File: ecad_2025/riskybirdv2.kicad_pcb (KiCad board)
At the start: 2 copper layers, 58.3 x 58.3 mm, 1 part

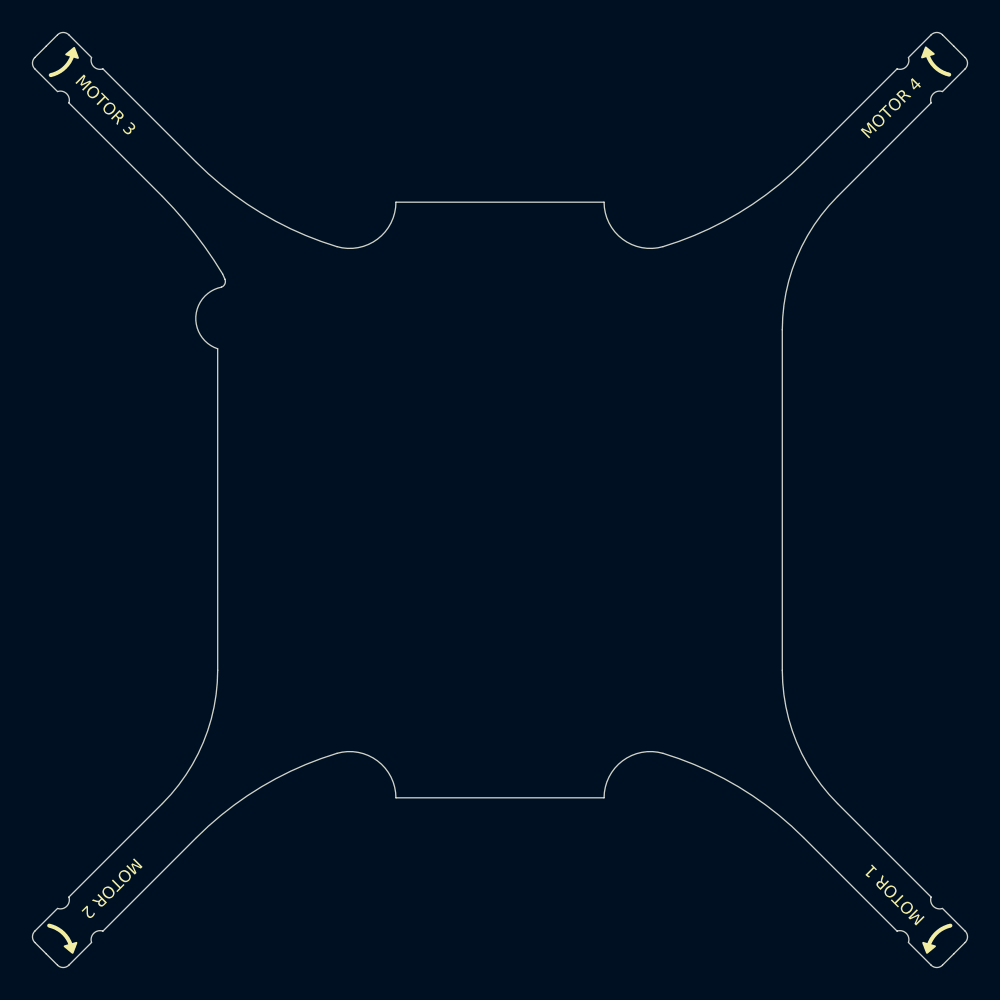
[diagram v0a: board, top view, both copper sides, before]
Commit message: first revision of riskybirdv2 sensor board
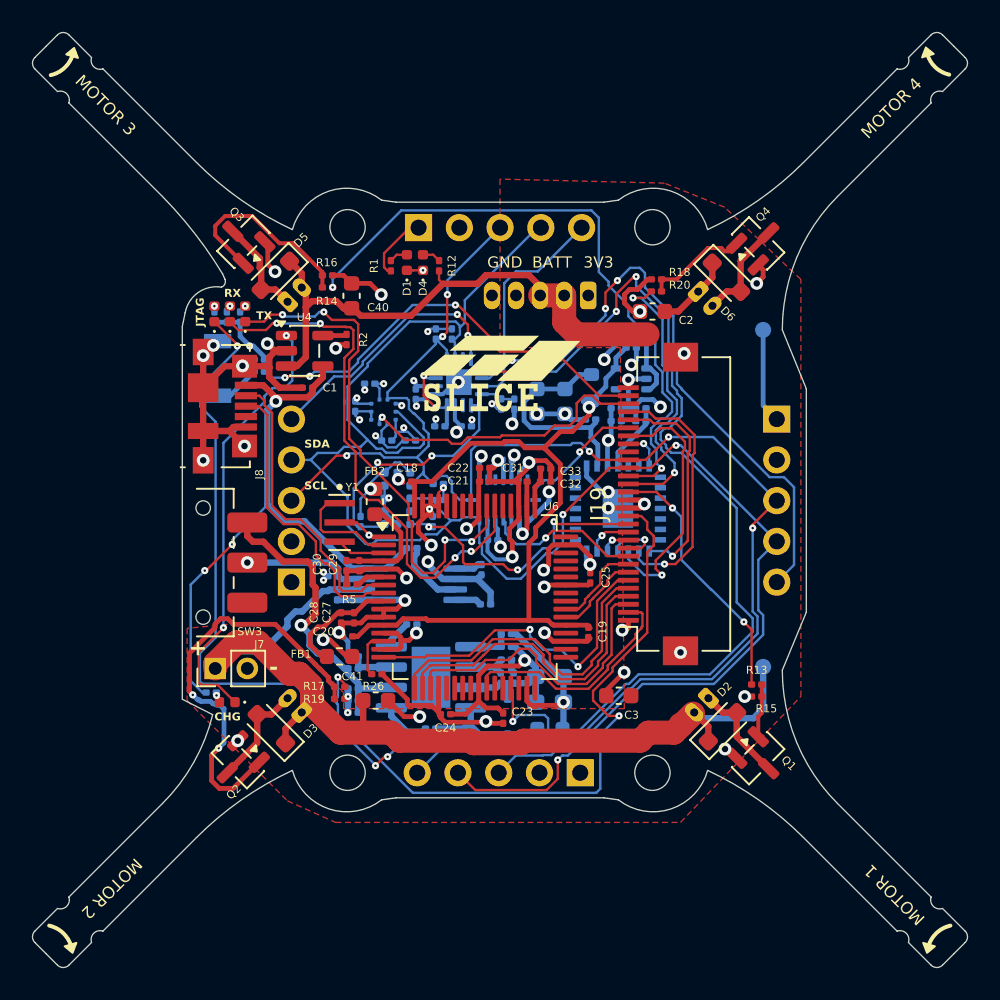
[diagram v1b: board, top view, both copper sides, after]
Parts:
- added C1: 4.7u, Capacitor_SMD:C_0201_0603Metric, F.Cu at (88.0, 93.0)
- added C10: 100nF, Capacitor_SMD:C_0201_0603Metric, B.Cu at (108.8, 95.1)
- added C11: 22uF, Capacitor_SMD:C_0603_1608Metric, B.Cu at (102.3, 93.9)
- added C12: 22uF, Capacitor_SMD:C_0603_1608Metric, B.Cu at (104.0, 93.9)
- added C13: 100nF, Capacitor_SMD:C_0201_0603Metric, B.Cu at (105.6, 95.0)
- added C14: 10uF, Capacitor_SMD:C_0201_0603Metric, B.Cu at (107.2, 95.1)
- added C15: 100nF, Capacitor_SMD:C_0201_0603Metric, B.Cu at (107.2, 94.3)
- added C16: 100n, Capacitor_SMD:C_0201_0603Metric, B.Cu at (91.0, 94.2)
- added C17: 100n, Capacitor_SMD:C_0201_0603Metric, B.Cu at (91.9, 92.8)
- added C18: 100nF, Capacitor_SMD:C_0201_0603Metric, F.Cu at (94.2, 98.8)
- added C19: 100nF, Capacitor_SMD:C_0201_0603Metric, F.Cu at (105.5, 108.2)
- added C2: 47uF, Capacitor_SMD:C_0603_1608Metric, F.Cu at (109.5, 88.2)
- added C20: 100nF, Capacitor_SMD:C_0201_0603Metric, F.Cu at (90.5, 108.5)
- added C21: 100nF, Capacitor_SMD:C_0201_0603Metric, F.Cu at (99.0, 98.8)
- added C22: 100nF, Capacitor_SMD:C_0201_0603Metric, F.Cu at (99.0, 98.0)
- added C23: 10uF, Capacitor_SMD:C_0201_0603Metric, F.Cu at (100.2, 113.6)
- added C24: 100nF, Capacitor_SMD:C_0201_0603Metric, F.Cu at (96.6, 113.3)
- added C25: 100nF, Capacitor_SMD:C_0201_0603Metric, F.Cu at (105.6, 104.8)
- added C26: 4.7u, Capacitor_SMD:C_0201_0603Metric, B.Cu at (89.8, 105.9)
- added C27: 100nF, Capacitor_SMD:C_0201_0603Metric, F.Cu at (90.9, 107.3)
- added C28: 4.7uF, Capacitor_SMD:C_0201_0603Metric, F.Cu at (90.1, 107.3)
- added C29: 100nF, Capacitor_SMD:C_0201_0603Metric, F.Cu at (91.2, 104.1)
- added C3: 47uF, Capacitor_SMD:C_0603_1608Metric, F.Cu at (107.4, 112.2)
- added C30: 4.7uF, Capacitor_SMD:C_0201_0603Metric, F.Cu at (90.4, 104.1)
- added C31: 100nF, Capacitor_SMD:C_0201_0603Metric, F.Cu at (101.4, 98.8)
- added C32: 3.3uF, Capacitor_SMD:C_0201_0603Metric, F.Cu at (102.8, 98.8)
- added C33: 100nF, Capacitor_SMD:C_0201_0603Metric, F.Cu at (102.8, 98.0)
- added C34: 1u, Capacitor_SMD:C_0201_0603Metric, B.Cu at (89.6, 104.8)
- added C38: 100nF, Capacitor_SMD:C_0201_0603Metric, B.Cu at (94.4, 96.3)
- added C39: 4.7uF, Capacitor_SMD:C_0201_0603Metric, B.Cu at (92.9, 96.3)
- added C4: 100nF, Capacitor_SMD:C_0201_0603Metric, B.Cu at (100.4, 97.5)
- added C40: 47uF, Capacitor_SMD:C_0603_1608Metric, F.Cu at (90.8, 87.3)
- added C41: 47uF, Capacitor_SMD:C_0603_1608Metric, F.Cu at (92.2, 112.5)
- added C42: 1uF, Capacitor_SMD:C_0201_0603Metric, B.Cu at (108.2, 90.5)
- added C47: 0.1uF, Capacitor_SMD:C_0201_0603Metric, B.Cu at (95.7, 114.2)
- added C48: 0.01uF, Capacitor_SMD:C_0201_0603Metric, B.Cu at (94.5, 107.8)
- added C49: 1000pF, Capacitor_SMD:C_0201_0603Metric, B.Cu at (100.0, 111.1)
- added C5: 100nF, Capacitor_SMD:C_0201_0603Metric, B.Cu at (99.5, 102.5)
- added C50: 47pF, Capacitor_SMD:C_0201_0603Metric, B.Cu at (100.4, 110.0)
- added C51: 4.7uF, Capacitor_SMD:C_0201_0603Metric, B.Cu at (90.8, 112.5)
- added C52: 47uF, Capacitor_SMD:C_0603_1608Metric_Pad1.08x0.95mm_HandSolder, B.Cu at (103.1, 112.6)
- added C53: 47uF, Capacitor_SMD:C_0603_1608Metric_Pad1.08x0.95mm_HandSolder, B.Cu at (103.1, 111.0)
- added C54: 0.01uF, Capacitor_SMD:C_0201_0603Metric, B.Cu at (90.8, 113.2)
- added C55: 4.7uF, Capacitor_SMD:C_0201_0603Metric, B.Cu at (90.8, 111.8)
- added C6: 100nF, Capacitor_SMD:C_0201_0603Metric, B.Cu at (97.9, 95.4)
- added C7: 100nF, Capacitor_SMD:C_0201_0603Metric, B.Cu at (94.8, 93.4)
- added C8: 1uF, Capacitor_SMD:C_0201_0603Metric, B.Cu at (96.2, 95.4)
- added C9: 4.7uF, Capacitor_SMD:C_0201_0603Metric, B.Cu at (108.8, 94.3)
- added D1: LED, LED_SMD:LED_0402_1005Metric, F.Cu at (94.2, 85.2)
- added D10: LED, LED_SMD:LED_0402_1005Metric, F.Cu at (83.2, 88.4)
- added D11: LED, LED_SMD:LED_0402_1005Metric, F.Cu at (84.1, 88.4)
- added D12: LED, LED_SMD:LED_0402_1005Metric, F.Cu at (82.2, 88.4)
- added D14: BAT54J, Diode_SMD:D_SOD-323F, B.Cu at (100.5, 113.5)
- added D2: BAT54JFILM, Diode_SMD:D_SOD-323_HandSoldering, F.Cu at (113.9, 114.1)
- added D3: BAT54JFILM, Diode_SMD:D_SOD-323_HandSoldering, F.Cu at (85.8, 114.2)
- added D4: LED, LED_SMD:LED_0402_1005Metric, F.Cu at (95.2, 85.2)
- added D5: BAT54JFILM, Diode_SMD:D_SOD-323_HandSoldering, F.Cu at (86.0, 86.0)
- added D6: BAT54JFILM, Diode_SMD:D_SOD-323_HandSoldering, F.Cu at (114.1, 86.1)
- added D7: LED_RED, LED_SMD:LED_0402_1005Metric, F.Cu at (83.0, 112.6)
- added FB1: 600R@100MHz/0.5A, Inductor_SMD:L_0603_1608Metric, F.Cu at (90.0, 109.8)
- added FB2: 600R@100MHz/0.5A, Inductor_SMD:L_0603_1608Metric, F.Cu at (92.2, 100.1)
- added G***: LOGO, LOGO, F.Cu at (100.0, 92.2)
- added G***: LOGO, LOGO, B.Cu at (108.2, 108.8)
- added G***: LOGO, LOGO, B.Cu at (113.8, 99.0)
- added G***: LOGO, LOGO, B.Cu at (92.2, 88.8)
- added H1: MountingHole, MountingHole:MountingHole_2.2mm_M2, F.Cu at (90.5, 83.0)
- added H2: MountingHole, MountingHole:MountingHole_2.2mm_M2, F.Cu at (109.5, 83.0)
- added H3: MountingHole, MountingHole:MountingHole_2.2mm_M2, F.Cu at (90.5, 117.0)
- added H4: MountingHole, MountingHole:MountingHole_2.2mm_M2, F.Cu at (109.5, 117.0)
- added IC1: PMW3901MB-TXQT, riskybird:PMW3901MBTXQT, B.Cu at (107.3, 100.5)
- added J10: Conn_01x05, Connector_PinHeader_2.54mm:PinHeader_1x05_P2.54mm_Vertical, B.Cu at (94.9, 83.0)
- added J11: Conn_01x05, Connector_PinHeader_2.54mm:PinHeader_1x05_P2.54mm_Vertical, B.Cu at (105.0, 117.0)
- added J18: Conn_01x05_MountingPin, Connector_JST:JST_ZH_B5B-ZR_1x05_P1.50mm_Vertical, B.Cu at (105.5, 87.2)
- added J19: Conn_01x30_MountingPin, Connector_FFC-FPC:Hirose_FH12-30S-0.5SH_1x30-1MP_P0.50mm_Horizontal, F.Cu at (109.8, 100.2)
- added J2: Conn_01x05, Connector_PinHeader_2.54mm:PinHeader_1x05_P2.54mm_Vertical, B.Cu at (117.2, 95.0)
- added J3: Conn_01x02, Connector_Molex:Molex_PicoBlade_53048-0210_1x02_P1.25mm_Horizontal, B.Cu at (113.0, 112.4)
- added J4: Conn_01x02, Connector_Molex:Molex_PicoBlade_53048-0210_1x02_P1.25mm_Horizontal, B.Cu at (86.8, 87.6)
- added J5: Conn_01x02, Connector_Molex:Molex_PicoBlade_53048-0210_1x02_P1.25mm_Horizontal, B.Cu at (87.6, 113.2)
- added J6: Conn_01x02, Connector_Molex:Molex_PicoBlade_53048-0210_1x02_P1.25mm_Horizontal, B.Cu at (112.4, 87.0)
- added J7: Conn_01x02, Connector_PinHeader_2.00mm:PinHeader_1x02_P2.00mm_Vertical, F.Cu at (82.2, 110.5)
- added J8: USB_B_Micro, Connector_USB:USB_Micro-B_Molex_47346-0001, F.Cu at (82.7, 94.2)
- added J9: Conn_01x05, Connector_PinHeader_2.54mm:PinHeader_1x05_P2.54mm_Vertical, B.Cu at (87.0, 105.1)
- added L3: 6.8uH, Inductor_SMD:L_0603_1608Metric, B.Cu at (103.1, 114.3)
- added Q1: SI2302, Package_TO_SOT_SMD:SOT-23, F.Cu at (116.1, 116.1)
- added Q2: SI2302, Package_TO_SOT_SMD:SOT-23, F.Cu at (83.7, 116.3)
- added Q3: SI2302, Package_TO_SOT_SMD:SOT-23, F.Cu at (84.0, 83.9)
- added Q4: SI2302, Package_TO_SOT_SMD:SOT-23, F.Cu at (116.1, 84.0)
- added R1: 150, Resistor_SMD:R_0201_0603Metric, F.Cu at (93.2, 85.4)
- added R12: 150, Resistor_SMD:R_0201_0603Metric, F.Cu at (96.2, 85.4)
- added R13: 47R, Resistor_SMD:R_0201_0603Metric, F.Cu at (116.0, 111.5)
- added R14: 47R, Resistor_SMD:R_0201_0603Metric, F.Cu at (89.2, 86.8)
- added R15: 10k, Resistor_SMD:R_0201_0603Metric, F.Cu at (116.0, 112.2)
- added R16: 10k, Resistor_SMD:R_0201_0603Metric, F.Cu at (89.2, 86.0)
- added R17: 47R, Resistor_SMD:R_0201_0603Metric, F.Cu at (90.0, 111.6)
- added R18: 47R, Resistor_SMD:R_0201_0603Metric, F.Cu at (109.8, 87.0)
- added R19: 10k, Resistor_SMD:R_0201_0603Metric, F.Cu at (90.0, 112.4)
- added R2: 2k, Resistor_SMD:R_0201_0603Metric, F.Cu at (90.4, 90.0)
- added R20: 10k, Resistor_SMD:R_0201_0603Metric, F.Cu at (109.8, 86.2)
- added R22: 4.7K, Resistor_SMD:R_0201_0603Metric, B.Cu at (97.0, 89.7)
- added R23: 4.7K, Resistor_SMD:R_0201_0603Metric, B.Cu at (96.0, 89.7)
- added R25: 3, Resistor_SMD:R_0603_1608Metric, B.Cu at (105.7, 93.0)
- added R26: 1k, Resistor_SMD:R_0201_0603Metric, F.Cu at (92.3, 110.8)
- added R27: 150, Resistor_SMD:R_0201_0603Metric, B.Cu at (83.0, 88.6)
- added R28: 150, Resistor_SMD:R_0201_0603Metric, B.Cu at (83.8, 88.6)
- added R29: 150, Resistor_SMD:R_0201_0603Metric, B.Cu at (82.2, 88.6)
- added R3: 150, Resistor_SMD:R_0201_0603Metric, B.Cu at (82.0, 112.0)
- added R30: 200K, Resistor_SMD:R_0201_0603Metric, B.Cu at (100.9, 94.0)
- added R31: 100K, Resistor_SMD:R_0201_0603Metric, B.Cu at (100.1, 94.0)
- added R32: 10K, Resistor_SMD:R_0201_0603Metric, B.Cu at (85.0, 91.2)
- added R33: 100, Resistor_SMD:R_0201_0603Metric, B.Cu at (85.0, 92.0)
- added R34: 10k, Resistor_SMD:R_0201_0603Metric, B.Cu at (94.5, 103.0)
- added R37: 150, Resistor_SMD:R_0201_0603Metric, B.Cu at (99.1, 106.5)
- added R38: 10k, Resistor_SMD:R_0201_0603Metric, B.Cu at (98.8, 104.3)
- added R41: 10k, Resistor_SMD:R_0201_0603Metric, B.Cu at (95.8, 101.3)
- added R42: 10k, Resistor_SMD:R_0201_0603Metric, B.Cu at (91.3, 101.3)
- added R43: 4.7K, Resistor_SMD:R_0201_0603Metric, B.Cu at (96.2, 100.0)
- added R44: 4.7K, Resistor_SMD:R_0201_0603Metric, B.Cu at (96.2, 99.0)
- added R45: 68.1k, Resistor_SMD:R_0201_0603Metric, B.Cu at (90.8, 109.8)
- added R46: 332k, Resistor_SMD:R_0201_0603Metric, B.Cu at (90.8, 110.5)
- added R47: 29.4k, Resistor_SMD:R_0201_0603Metric, B.Cu at (100.8, 111.1)
- added R48: 10.2k, Resistor_SMD:R_0201_0603Metric, B.Cu at (100.4, 108.3)
- added R49: 3.24k, Resistor_SMD:R_0201_0603Metric, B.Cu at (100.4, 109.2)
- added R5: 12k, Resistor_SMD:R_0201_0603Metric, F.Cu at (90.8, 105.2)
- added SW2: SW_SPST, Button_Switch_SMD:SW_SPST_B3U-1000P, B.Cu at (82.4, 91.8)
- added SW3: SW_SPST, Button_Switch_SMD:SW_SPDT_CK_JS102011SAQN, F.Cu at (81.5, 103.9)
- added TP1: TestPoint, TestPoint:TestPoint_Pad_D1.0mm, B.Cu at (116.4, 110.4)
- added TP6: TestPoint, TestPoint:TestPoint_Pad_D1.0mm, B.Cu at (116.4, 89.4)
- added U1: ADS7128IRTER, Package_DFN_QFN:WQFN-16-1EP_3x3mm_P0.5mm_EP1.6x1.6mm, B.Cu at (97.4, 92.7)
- added U10: TLV70018DCKR, Package_TO_SOT_SMD:SOT-353_SC-70-5, B.Cu at (108.2, 92.5)
- added U11: TPS54331D, Package_SO:SOIC-8-1EP_3.9x4.9mm_P1.27mm_EP2.41x3.81mm, B.Cu at (95.7, 111.0)
- added U3: BMI088, Package_LGA:Bosch_LGA-16_4.5x3mm_P0.5mm_LayoutBorder7x1y_ClockwisePinNumbering, B.Cu at (100.2, 100.0)
- added U4: MCP73831-2-OT, Package_TO_SOT_SMD:SOT-23-5, F.Cu at (87.8, 90.7)
- added U5: ~, riskybird:BMP390, B.Cu at (92.7, 94.5)
- added U6: FT2232HL-REEL, Package_QFP:LQFP-64_10x10mm_P0.5mm, F.Cu at (98.4, 106.0)
- added U7: TPS2113A, Package_SO:TSSOP-8_4.4x3mm_P0.65mm, B.Cu at (94.3, 105.2)
- added U9: VL53L1CXV0FY1, Sensor_Distance:ST_VL53L1x, B.Cu at (93.6, 99.9)
- added Y1: f, riskybird:OSC_CSTNE12M0G550000R0, F.Cu at (90.0, 101.4)
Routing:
- net GND: track 0.00 -> 163.2 mm, vias 0 -> 57
- net /SDA: track 0.00 -> 112.2 mm, vias 0 -> 3
- net +BATT: track 0.00 -> 100.0 mm
- net +3V3: track 0.00 -> 91.7 mm, vias 0 -> 23
- net /SCL: track 0.00 -> 90.9 mm, vias 0 -> 6
- net /GPIO3: track 0.00 -> 64.2 mm, vias 0 -> 4
- net /JTAG_LED: track 0.00 -> 55.8 mm, vias 0 -> 4
- net +1V8: track 0.00 -> 47.9 mm, vias 0 -> 1
- net /MOTOR2: track 0.00 -> 43.0 mm, vias 0 -> 2
- net /MOTOR3: track 0.00 -> 39.8 mm, vias 0 -> 2
- net +5V: track 0.00 -> 38.3 mm, vias 0 -> 3
- net /GPIO2: track 0.00 -> 37.9 mm, vias 0 -> 4
- net /RX_LED: track 0.00 -> 33.9 mm, vias 0 -> 4
- net /TX_LED: track 0.00 -> 32.7 mm, vias 0 -> 4
- net Net-(D7-K): track 0.00 -> 27.4 mm, vias 0 -> 2
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- added copper zone on In2.Cu, net +3V3
- added copper zone on F.Cu, net +BATT
- added copper zone on In1.Cu, net GND
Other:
- outline, holes or cut-outs redrawn
- copper layers 2 -> 4
- board text added: "+"
- board text added: "-"
- board text added: "3V3"
- board text added: "BATT"
- board text added: "CHG"
- board text added: "GND"
- board text added: "JTAG"
- board text added: "RX"
- board text added: "SCL"
- board text added: "SDA"
- board text added: "TX"
- board text added: "V2"
